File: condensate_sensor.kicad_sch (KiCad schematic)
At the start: 3 parts

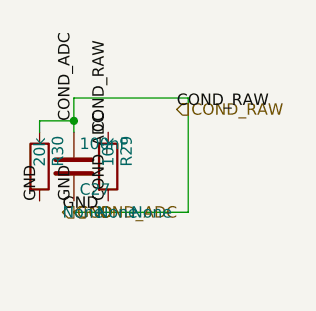
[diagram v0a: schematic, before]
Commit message: all unit test pass
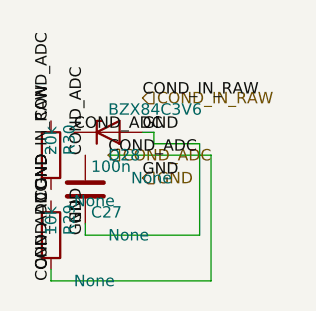
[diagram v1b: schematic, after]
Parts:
- added D28: BZX84C3V6, symbol Device:D_Zener
- C27: value 100nF -> 100n
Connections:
- net COND_ADC: now also D28.1 (K)
- net GND: now also D28.2 (A)
- net COND_RAW renamed COND_IN_RAW
